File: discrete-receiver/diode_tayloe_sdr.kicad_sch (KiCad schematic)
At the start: 9 parts, among them J5 Display Connector, X1 YC24.576MUBCE2O

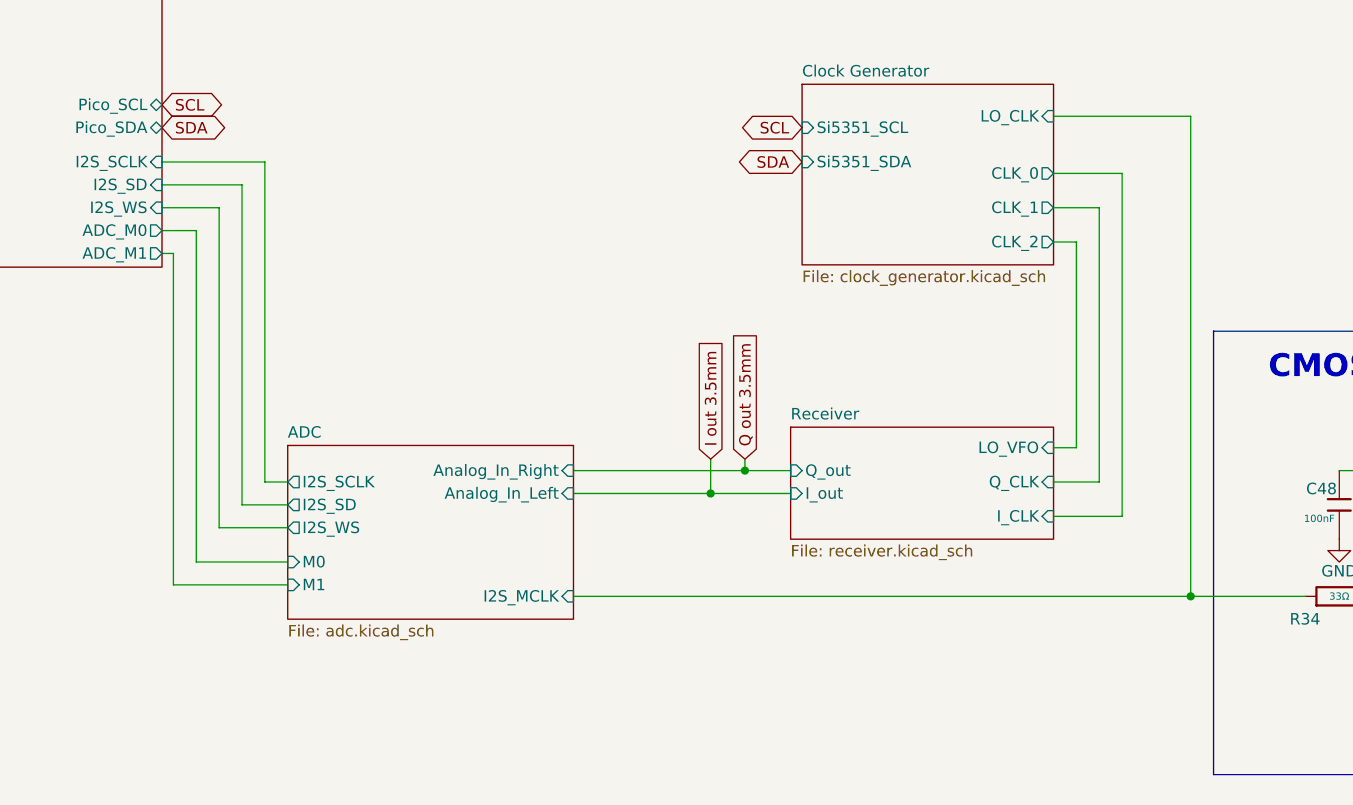
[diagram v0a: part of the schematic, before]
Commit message: Made ERC progress
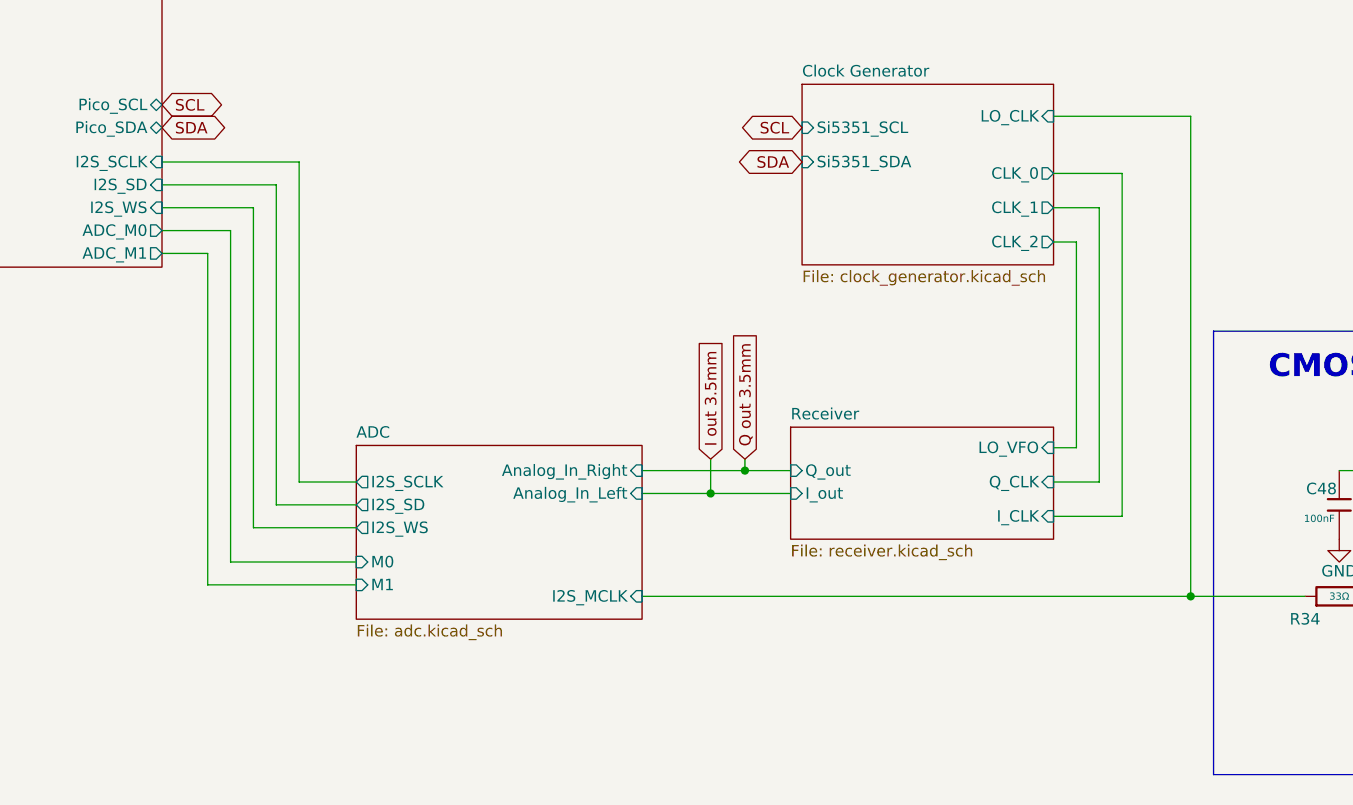
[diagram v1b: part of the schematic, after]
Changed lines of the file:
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@@
 	)
 	(junction
-		(at 45.72 53.34)
+		(at 181.61 133.35)
 		(diameter 0)
 		(color 0 0 0 0)
 	)
 	(junction
-		(at 55.88 39.37)
+		(at 45.72 53.34)
 		(diameter 0)
 		(color 0 0 0 0)
 	)
 	(junction
-		(at 33.02 72.39)
+		(at 55.88 39.37)
 		(diameter 0)
 		(color 0 0 0 0)
 	)
 	(junction
-		(at 234.95 144.78)
+		(at 33.02 72.39)
 		(diameter 0)
 		(color 0 0 0 0)
@@
 	)
 	(junction
-		(at 45.72 48.26)
+		(at 234.95 144.78)
 		(diameter 0)
 		(color 0 0 0 0)
 	)
 	(junction
-		(at 185.42 130.81)
+		(at 45.72 48.26)
 		(diameter 0)
 		(color 0 0 0 0)
 	)
 	(junction
-		(at 181.61 133.35)
+		(at 259.08 130.81)
 		(diameter 0)
 		(color 0 0 0 0)
 	)
 	(junction
-		(at 259.08 130.81)
+		(at 185.42 130.81)
 		(diameter 0)
 		(color 0 0 0 0)
@@
 	(wire
 		(pts
-			(xy 120.65 104.14) (xy 124.46 104.14)
+			(xy 120.65 104.14) (xy 128.27 104.14)
 		)
 		(stroke
@@
 	(wire
 		(pts
-			(xy 124.46 140.97) (xy 134.62 140.97)
+			(xy 128.27 140.97) (xy 142.24 140.97)
 		)
 		(stroke
@@
 	(wire
 		(pts
-			(xy 166.37 133.35) (xy 181.61 133.35)
+			(xy 173.99 133.35) (xy 181.61 133.35)
 		)
 		(stroke
@@
 	(wire
 		(pts
-			(xy 121.92 143.51) (xy 121.92 106.68)
+			(xy 125.73 143.51) (xy 125.73 106.68)
 		)
 		(stroke
@@
 	(wire
 		(pts
-			(xy 127 137.16) (xy 134.62 137.16)
+			(xy 130.81 137.16) (xy 142.24 137.16)
 		)
 		(stroke
@@
 	(wire
 		(pts
-			(xy 120.65 101.6) (xy 127 101.6)
+			(xy 120.65 101.6) (xy 130.81 101.6)
 		)
 		(stroke
@@
 	(wire
 		(pts
-			(xy 124.46 104.14) (xy 124.46 140.97)
+			(xy 128.27 104.14) (xy 128.27 140.97)
 		)
 		(stroke
@@
 	(wire
 		(pts
-			(xy 121.92 106.68) (xy 120.65 106.68)
+			(xy 125.73 106.68) (xy 120.65 106.68)
 		)
 		(stroke
@@
 	(wire
 		(pts
-			(xy 134.62 143.51) (xy 121.92 143.51)
+			(xy 142.24 143.51) (xy 125.73 143.51)
 		)
 		(stroke
@@
 	(wire
 		(pts
-			(xy 127 101.6) (xy 127 137.16)
+			(xy 130.81 101.6) (xy 130.81 137.16)
 		)
 		(stroke
@@
 	(wire
 		(pts
-			(xy 120.65 96.52) (xy 132.08 96.52)
+			(xy 120.65 96.52) (xy 135.89 96.52)
 		)
 		(stroke
@@
 	(wire
 		(pts
-			(xy 129.54 134.62) (xy 134.62 134.62)
+			(xy 133.35 134.62) (xy 142.24 134.62)
 		)
 		(stroke
@@
 	(wire
 		(pts
-			(xy 166.37 144.78) (xy 234.95 144.78)
+			(xy 173.99 144.78) (xy 234.95 144.78)
 		)
 		(stroke
@@
 	(wire
 		(pts
-			(xy 166.37 130.81) (xy 185.42 130.81)
+			(xy 173.99 130.81) (xy 185.42 130.81)
 		)
 		(stroke
@@
 	(wire
 		(pts
-			(xy 132.08 132.08) (xy 134.62 132.08)
+			(xy 135.89 132.08) (xy 142.24 132.08)
 		)
 		(stroke
@@
 	(wire
 		(pts
-			(xy 129.54 99.06) (xy 129.54 134.62)
+			(xy 133.35 99.06) (xy 133.35 134.62)
 		)
 		(stroke
@@
 	(wire
 		(pts
-			(xy 132.08 96.52) (xy 132.08 132.08)
+			(xy 135.89 96.52) (xy 135.89 132.08)
 		)
 		(stroke
@@
 	(wire
 		(pts
-			(xy 120.65 99.06) (xy 129.54 99.06)
+			(xy 120.65 99.06) (xy 133.35 99.06)
 		)
 		(stroke
@@
 	)
 	(sheet
-		(at 134.62 128.016)
+		(at 142.24 128.016)
 		(size 31.75 19.304)
 		(exclude_from_sim no)
@@
 		)
 		(property "Sheetname" "ADC"
-			(at 134.62 127.3044 0)
+			(at 142.24 127.3044 0)
 			(show_name no)
 			(do_not_autoplace no)
@@
 		)
 		(property "Sheetfile" "adc.kicad_sch"
-			(at 134.62 147.9046 0)
+			(at 142.24 147.9046 0)
 			(show_name no)
 			(do_not_autoplace no)
@@
 		)
 		(pin "Analog_In_Left" input
-			(at 166.37 133.35 0)
+			(at 173.99 133.35 0)
 			(effects
 				(font
@@
 		)
 		(pin "Analog_In_Right" input
-			(at 166.37 130.81 0)
+			(at 173.99 130.81 0)
 			(effects
 				(font
@@
 		)
 		(pin "I2S_MCLK" input
-			(at 166.37 144.78 0)
+			(at 173.99 144.78 0)
 			(effects
 				(font
@@
 		)
 		(pin "I2S_SCLK" output
-			(at 134.62 132.08 180)
+			(at 142.24 132.08 180)
 			(effects
 				(font
@@
 		)
 		(pin "I2S_SD" output
-			(at 134.62 134.62 180)
+			(at 142.24 134.62 180)
 			(effects
 				(font
@@
 		)
 		(pin "I2S_WS" output
-			(at 134.62 137.16 180)
+			(at 142.24 137.16 180)
 			(effects
 				(font
@@
 		)
 		(pin "M0" input
-			(at 134.62 140.97 180)
+			(at 142.24 140.97 180)
 			(effects
 				(font
@@
 		)
 		(pin "M1" input
-			(at 134.62 143.51 180)
+			(at 142.24 143.51 180)
 			(effects
 				(font
